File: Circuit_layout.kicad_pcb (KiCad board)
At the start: 2 copper layers, 203.2 x 165.1 mm, 249 parts, among them IC1 TS431ILT, IC4 TS431ILT, J1 TSV, J10 CoolingPower, J13 Cooling_RTN, J18 ICSP, J2 CoolingSystem, J21 Lights On Car, J24 Cockpit, J25 RJ11, J3 Pedal, J32 Conn_MC, J34 Can_Iso, J35 GLV_In, J36 GLV_Out, J4 Conn_01x08, J5 Testing Connector, J6 AIRs/SafetyLoop, J7 IMD, J8 DC_Relay, J9 PC_Relay, K1 APAN3105, K2 G6B-1174P-US-DC24, K4 G6B-1174P-US-DC24, Q1 ZVP0545G, Q2 MMBF170, Q3 ZVP1320F, Q4 STN3NF06L, Q5 SI1302DL-T1-E3, Q8 SI1302DL-T1-E3, SW2 TS5A3159-Q1, SW4 SW_PUSH, U1 RDE03110S12, U10 MCP2551-I/SN, U11 TLP293, U12 TLP293, U13 REF3033, U14 Mounting_hole, U15 Mounting_hole, U16 MCP9700AT-H/TT, U17 Chassis Ground, U18 TS912, U19 74HC00, U2 MCP6002, U20 MC7805BDTRKG, U21 MCP6004, U22 TS372, U23 TLP293, U24 TLP293, U25 NCD9830DBR2G, U26 MCP6004, U27 TLP293, U28 Mounting_hole, U3 MCP6004, U30 DAC5574IDGS, U31 TLP293, U32 TLP293, U37 TLP293, U4 ACPL-C870, U40 MCP6004, U41 PDQ10-Q24-D5-D, U42 LT1763CS8-3.3PBF, U5 SI8600AB-B-IS, U6 TS912, U7 MCP23016, U8 74ACT11030, U9 PIC32MZ2048EFM064-I/PT

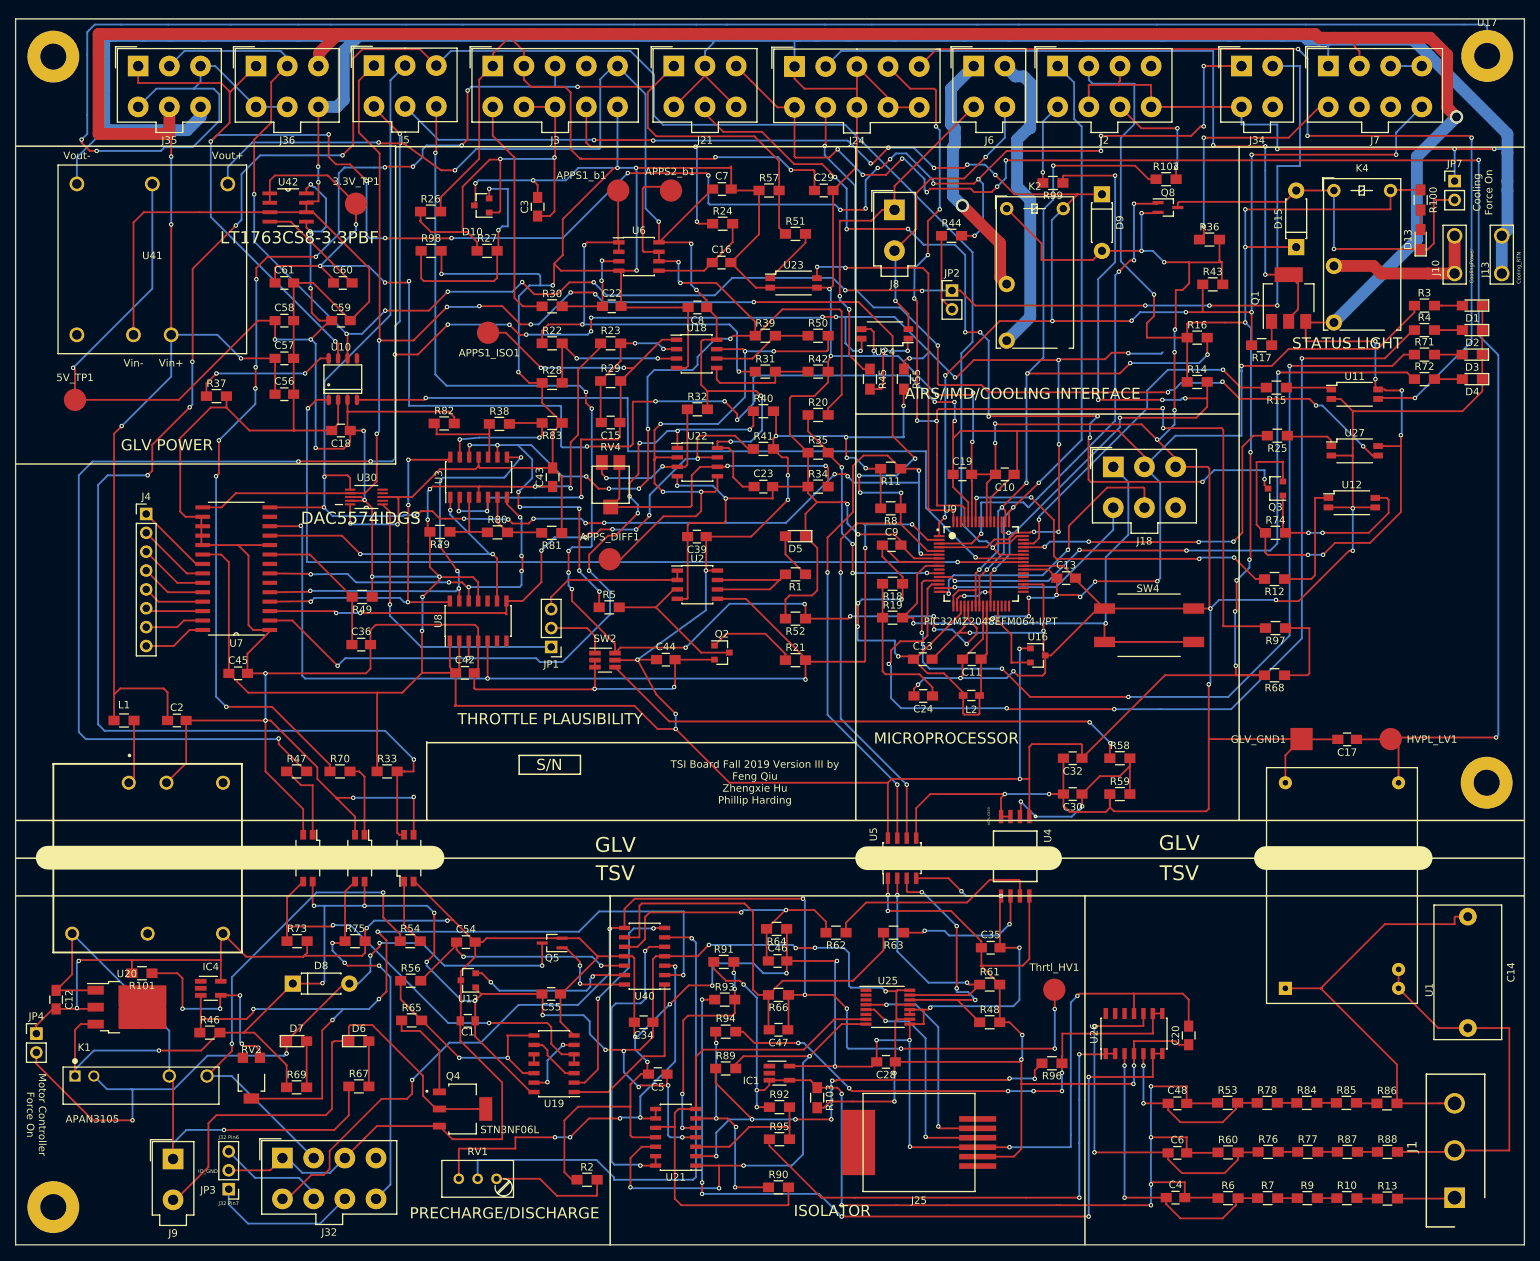
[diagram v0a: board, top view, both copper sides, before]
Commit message: TSI v4.1
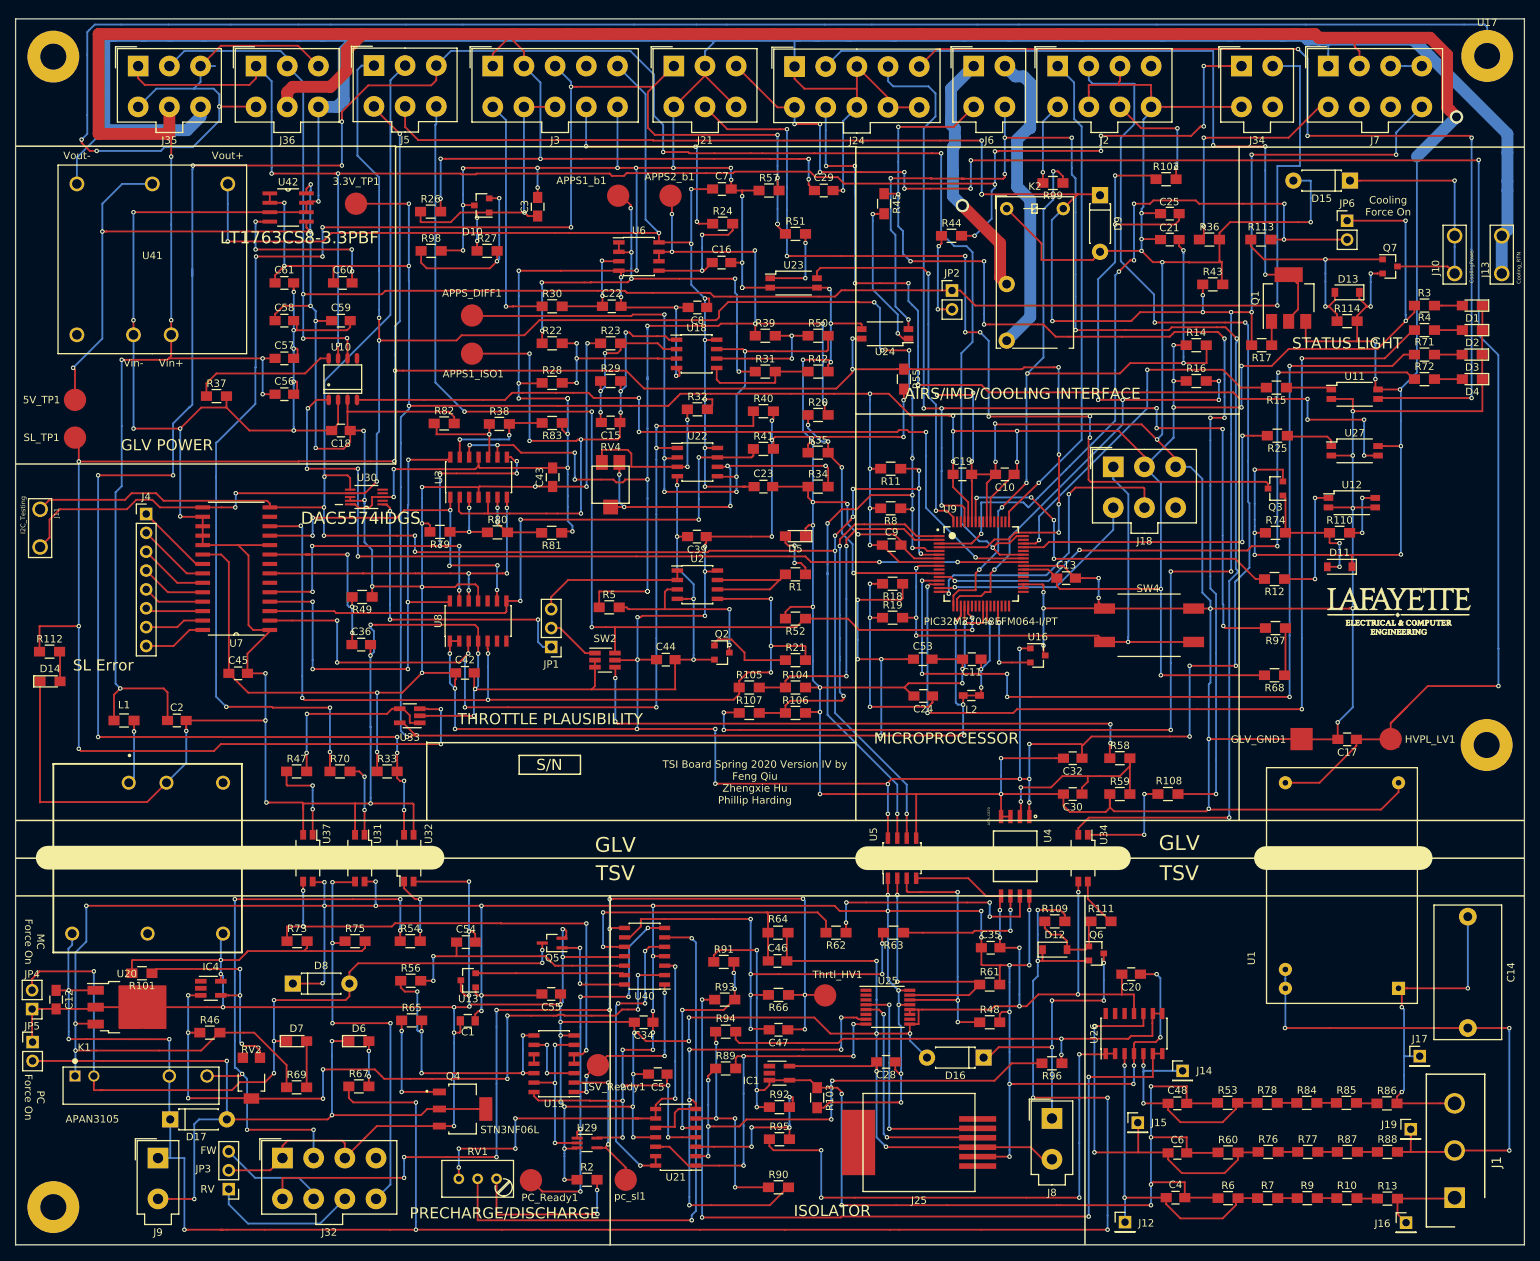
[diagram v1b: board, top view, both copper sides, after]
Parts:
- removed JP7: Jumper-Device, Pin_Headers:Pin_Header_Straight_1x02_Pitch2.54mm
- removed K4: G6B-1174P-US-DC24, custom_footprints:Relay_SPST_Finder_32.21-x300_special
- removed Q8: SI1302DL-T1-E3, custom_footprints:SOT-323_SC-70_Handsoldering_special
- removed R100: 500, Resistors_SMD:R_0805_HandSoldering
- added C21: 0.1u, Capacitors_SMD:C_0805_HandSoldering, F.Cu at (210.1, 58.9)
- added C25: 0.1u, Capacitors_SMD:C_0805_HandSoldering, F.Cu at (210.1, 55.4)
- added D11: MMSZ5231B-7-F, Diodes_SMD:D_SOD-123, F.Cu at (232.9, 103.0)
- added D12: MMSZ5231B-7-F, Diodes_SMD:D_SOD-123, F.Cu at (194.6, 154.6)
- added D14: SL Error, LEDs:LED_0805_HandSoldering, F.Cu at (59.2, 118.4)
- added D16: 1N4001, Diodes_THT:D_DO-41_SOD81_P7.62mm_Horizontal, F.Cu at (185.0, 169.1)
- added D17: 1N4001, Diodes_THT:D_DO-41_SOD81_P7.62mm_Horizontal, F.Cu at (75.4, 177.4)
- added G***: LOGO, QR:QR_500, B.Cu at (248.0, 108.8)
- added G***: LOGO, custom_footprints:logo_lafayette_ece_20mmx7mm, F.Cu at (240.9, 109.2)
- added J11: I2C_Testing, 1217861-1:TE_1217861-1, F.Cu at (57.9, 97.8)
- added J12: Conn_01x01, Pin_Headers:Pin_Header_Straight_1x01_Pitch2.54mm, F.Cu at (204.0, 191.3)
- added J14: Conn_01x01, Pin_Headers:Pin_Header_Straight_1x01_Pitch2.54mm, F.Cu at (211.8, 170.9)
- added J15: Conn_01x01, Pin_Headers:Pin_Header_Straight_1x01_Pitch2.54mm, F.Cu at (205.7, 177.9)
- added J16: Conn_01x01, Pin_Headers:Pin_Header_Straight_1x01_Pitch2.54mm, F.Cu at (241.9, 191.3)
- added J17: Conn_01x01, Pin_Headers:Pin_Header_Straight_1x01_Pitch2.54mm, F.Cu at (243.7, 168.9)
- added J19: Conn_01x01, Pin_Headers:Pin_Header_Straight_1x01_Pitch2.54mm, F.Cu at (242.5, 178.8)
- added JP5: Jumper-Device, Pin_Headers:Pin_Header_Straight_1x02_Pitch2.54mm, F.Cu at (56.9, 167.0)
- added JP6: Jumper, Pin_Headers:Pin_Header_Straight_1x02_Pitch2.54mm, F.Cu at (233.9, 56.4)
- added PC_Ready1: Precharge_Ready, Measurement_Points:Measurement_Point_Round-SMD-Pad_Big, F.Cu at (124.0, 185.6)
- added Q6: ZVP1320F, TO_SOT_Packages_SMD:SOT-23, F.Cu at (200.2, 155.1)
- added Q7: ZVP1320F, TO_SOT_Packages_SMD:SOT-23, F.Cu at (239.7, 62.5)
- added R104: 1k, Resistors_SMD:R_0805_HandSoldering, F.Cu at (159.6, 119.3)
- added R105: 500, Resistors_SMD:R_0805_HandSoldering, F.Cu at (153.4, 119.3)
- added R106: 500, Resistors_SMD:R_0805_HandSoldering, F.Cu at (159.6, 122.7)
- added R107: 3k, Resistors_SMD:R_0805_HandSoldering, F.Cu at (153.4, 122.7)
- added R108: 2.4k, Resistors_SMD:R_0805_HandSoldering, F.Cu at (209.8, 133.6)
- added R109: 1M, Resistors_SMD:R_0805_HandSoldering, F.Cu at (194.6, 150.7)
- added R110: 10k, Resistors_SMD:R_0805_HandSoldering, F.Cu at (232.9, 98.4)
- added R111: 10k, Resistors_SMD:R_0805_HandSoldering, F.Cu at (200.8, 150.7)
- added R112: 330, Resistors_SMD:R_0805_HandSoldering, F.Cu at (59.2, 114.4)
- added R113: 10k, Resistors_SMD:R_0805_HandSoldering, F.Cu at (222.3, 58.9)
- added R114: 1M, Resistors_SMD:R_0805_HandSoldering, F.Cu at (233.9, 69.9)
- added SL_TP1: SL_TP, Measurement_Points:Measurement_Point_Round-SMD-Pad_Big, F.Cu at (62.6, 85.6)
- added TSV_Ready1: TSV_Ready, Measurement_Points:Measurement_Point_Round-SMD-Pad_Big, F.Cu at (133.0, 170.1)
- added U29: SN74LVC1G08DCKR, TO_SOT_Packages_SMD:SOT-353_SC-70-5_Handsoldering, F.Cu at (131.6, 180.6)
- added U33: MCP6001, TO_SOT_Packages_SMD:SOT-23-5_HandSoldering, F.Cu at (107.7, 123.1)
- added U34: TLP293, Housings_SSOP:SOP-4_4.4x2.8mm_Pitch1.27mm, F.Cu at (198.4, 142.2)
- added pc_sl1: pc_sl, Measurement_Points:Measurement_Point_Round-SMD-Pad_Big, F.Cu at (136.8, 185.5)
- D13: value LED -> MMSZ5231B-7-F; footprint LEDs:LED_0805_HandSoldering -> Diodes_SMD:D_SOD-123
- R74: value 2.4K -> 1M
- U1: footprint custom_footprints:RDE03110S12 -> custom_footprints:RDE03110S12_new
- moved J8 124.2 mm to (194.2, 177.3)
- moved APPS_DIFF1 37.7 mm to (116.1, 69.2)
- moved Thrtl_HV1 30.9 mm to (163.6, 160.7)
- moved R45 23.7 mm to (171.6, 54.1)
- moved D13 12.2 mm to (233.9, 66.0), turned to 180 degrees
- moved D15 11.5 mm to (234.3, 51.0), turned to 180 degrees
- moved C20 11.3 mm to (204.9, 157.9), turned to 180 degrees
- moved R16 5.84 mm to (213.6, 78.0)
- moved U14 5.08 mm to (252.7, 127.0)
- moved R14 4.95 mm to (213.6, 73.2)
- moved APPS1_ISO1 3.55 mm to (116.1, 74.3)
- moved JP4 3.35 mm to (56.8, 162.6), turned to 180 degrees
- moved J9 2.04 mm to (73.8, 182.6)
- moved APPS2_b1 0.70 mm to (142.8, 53.0)
- moved APPS1_b1 0.70 mm to (135.8, 53.0)
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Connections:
- D13 pad 1: Net-(D13-Pad1) -> /+24V
- D15 pad 1: /+5V -> /Cooling_power
- D15 pad 2: Net-(D13-Pad1) -> /BP_RTN
- J36 pad 3: /+24V -> /CH_gnd
- J36 pad 5: /CH_gnd -> /+24V
- J8 pad 1: /AIRs+ -> /Pre-Charge/DC_Relay+
- J8 pad 2: /AIRs- -> /I/O_Ground
- Q3 pad 1: Net-(Q3-Pad1) -> Net-(D11-Pad2)
- R102 pad 1: /CoolTemp_1 -> /CoolTemp_2
- R11 pad 2: /+5V -> /+3.3V
- R14 pad 1: /+5V -> /+3.3V
- R14 pad 2: /CoolTemp_2 -> /CoolTemp_1
- R16 pad 1: /+5V -> /+3.3V
- R16 pad 2: /CoolTemp_1 -> /CoolTemp_2
- R47 pad 2: /Safety_Loop -> Net-(R47-Pad2)
- R68 pad 2: /+5V -> /+3.3V
- R74 pad 2: Net-(Q3-Pad1) -> Net-(D11-Pad2)
- R8 pad 2: /+5V -> /+3.3V
- R99 pad 1: /CoolTemp_2 -> /CoolTemp_1
- U12 pad 4: Net-(Q3-Pad1) -> Net-(R110-Pad2)
- U19 pad 2: /Pre-Charge/Precharge_Ready -> /Pre-Charge/pc_and_sl_ready
- U20 pad 4: (no net) -> /I/O_Ground
- U5 pad 6: /SDA -> /SCL
- U5 pad 7: /SCL -> /SDA
- U9 pad 1: /IMD_Status -> /IMD_Status_3.3
- U9 pad 2: /Throttle_PL -> /Throttle_PL_3.3
- U9 pad 23: /CoolTemp_1 -> Net-(U9-Pad23)
- U9 pad 24: /FlowRate -> Net-(U9-Pad24)
- U9 pad 27: /CoolTemp_2 -> Net-(U9-Pad27)
- U9 pad 50: /CoolTemp_1 -> Net-(U9-Pad50)
- U9 pad 51: /CoolTemp_2 -> Net-(U9-Pad51)
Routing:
- net /Pre-Charge/+24HV: track 81.1 -> 282.5 mm, vias 1 -> 11
- net /+3.3V: track 398.3 -> 577.7 mm, vias 24 -> 34
- net /AIRs-: track 40.0 -> 191.3 mm, vias 2 -> 8
- net /AIRs+: track 48.5 -> 153.3 mm, vias 2 -> 9
- net /BP_RTN: track 1628.4 -> 1722.5 mm, vias 52 -> 97
- net /IMD_Status: track 243.8 -> 337.2 mm
- net /+5V: track 764.0 -> 692.1 mm, vias 39 -> 47
- net /+5HV: track 376.4 -> 446.3 mm, vias 25 -> 40
- net /I/O_Ground: track 454.0 -> 512.2 mm, vias 20 -> 35
- net Net-(D13-Pad1): track 52.9 -> 0.00 mm, vias 1 -> 0
- net /IMD_Status_3.3: track 0.00 -> 49.3 mm, vias 0 -> 2
- net /Throttle_PL_3.3: track 0.00 -> 45.2 mm, vias 0 -> 2
- net /Pre-Charge/DC_Relay+: track 0.00 -> 39.4 mm, vias 0 -> 4
- net /GLV Interface/CAN_H: track 253.2 -> 217.4 mm, vias 19 -> 10
- net /+24V: track 549.6 -> 585.2 mm, vias 13 -> 22
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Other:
- board text added: "FW"
- board text added: "MC Force On"
- board text added: "PC Force On"
- board text added: "RV"
- board text added: "SL Error"
- board text added: "TSI Board Spring 2020 Version IV by Feng Qiu Zhengxie Hu Phillip Harding"
- board text removed: "IO_GND"
- board text removed: "J32 Pin6"
- board text removed: "J32 Pin7"
- board text removed: "Motor Controller Force On"
- board text removed: "TSI Board Fall 2019 Version III by Feng Qiu Zhengxie Hu Phillip Harding"
